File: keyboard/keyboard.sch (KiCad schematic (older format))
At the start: 356 parts, among them K1 KEYSW, K10 KEYSW, K100 KEYSW, K101 KEYSW, K102 KEYSW, K103 KEYSW, K104 KEYSW, K11 KEYSW, K12 KEYSW, K13 KEYSW, K14 KEYSW, K15 KEYSW, K16 KEYSW, K17 KEYSW, K18 KEYSW, K19 KEYSW, K2 KEYSW, K20 KEYSW, K21 KEYSW, K22 KEYSW, K23 KEYSW, K24 KEYSW, K25 KEYSW, K26 KEYSW, K27 KEYSW, K28 KEYSW, K29 KEYSW, K3 KEYSW, K30 KEYSW, K31 KEYSW, K32 KEYSW, K33 KEYSW, K34 KEYSW, K35 KEYSW, K36 KEYSW, K37 KEYSW, K38 KEYSW, K39 KEYSW, K4 KEYSW, K40 KEYSW, K41 KEYSW, K42 KEYSW, K43 KEYSW, K44 KEYSW, K45 KEYSW, K46 KEYSW, K47 KEYSW, K48 KEYSW, K49 KEYSW, K5 KEYSW, K50 KEYSW, K51 KEYSW, K52 KEYSW, K53 KEYSW, K54 KEYSW, K55 KEYSW, K56 KEYSW, K57 KEYSW, K58 KEYSW, K59 KEYSW, K6 KEYSW, K60 KEYSW, K61 KEYSW, K62 KEYSW, K63 KEYSW, K64 KEYSW, K65 KEYSW, K66 KEYSW, K67 KEYSW, K68 KEYSW, K69 KEYSW, K7 KEYSW, K70 KEYSW, K71 KEYSW, K72 KEYSW, K73 KEYSW, K74 KEYSW, K75 KEYSW, K76 KEYSW, K77 KEYSW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

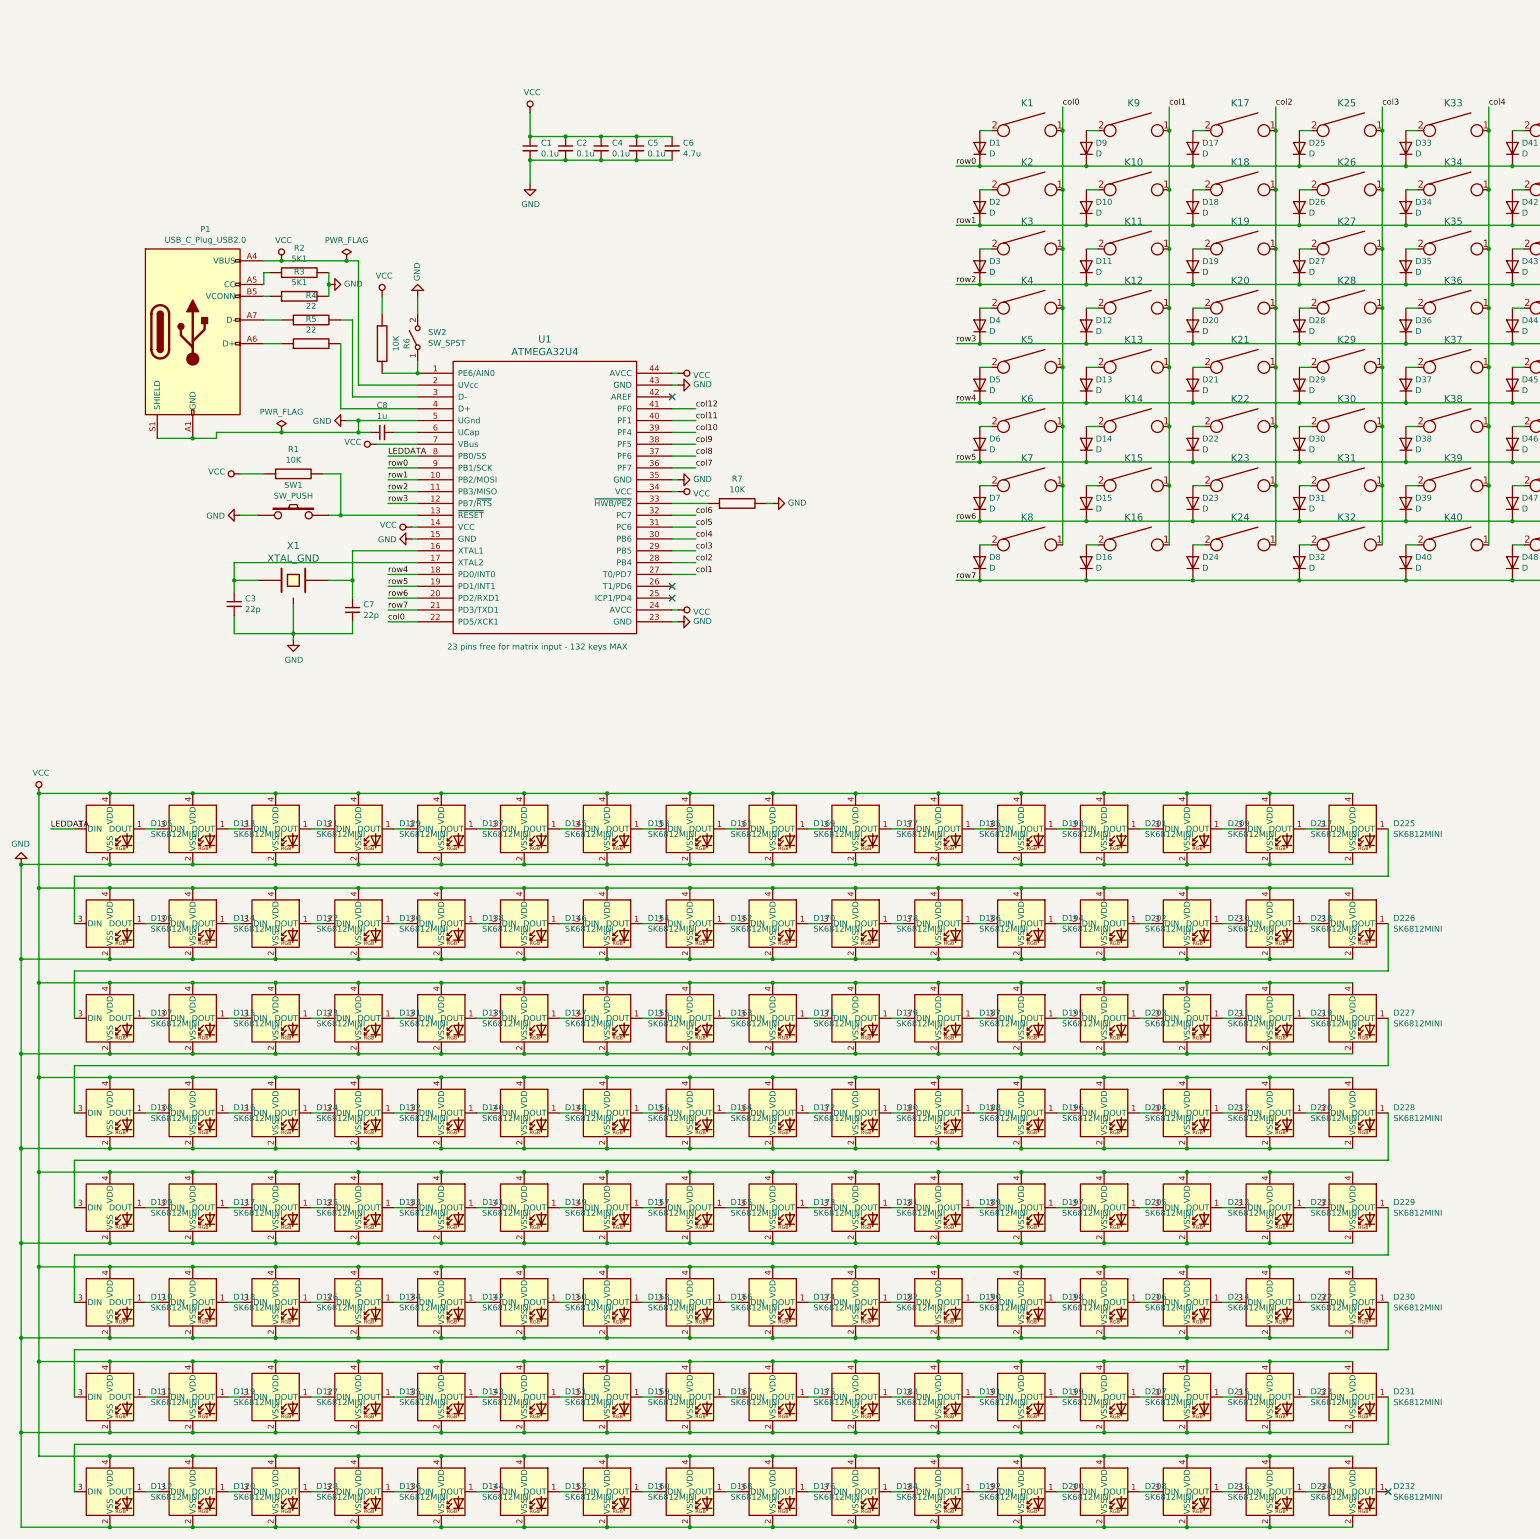
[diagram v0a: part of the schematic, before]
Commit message: add datasheets
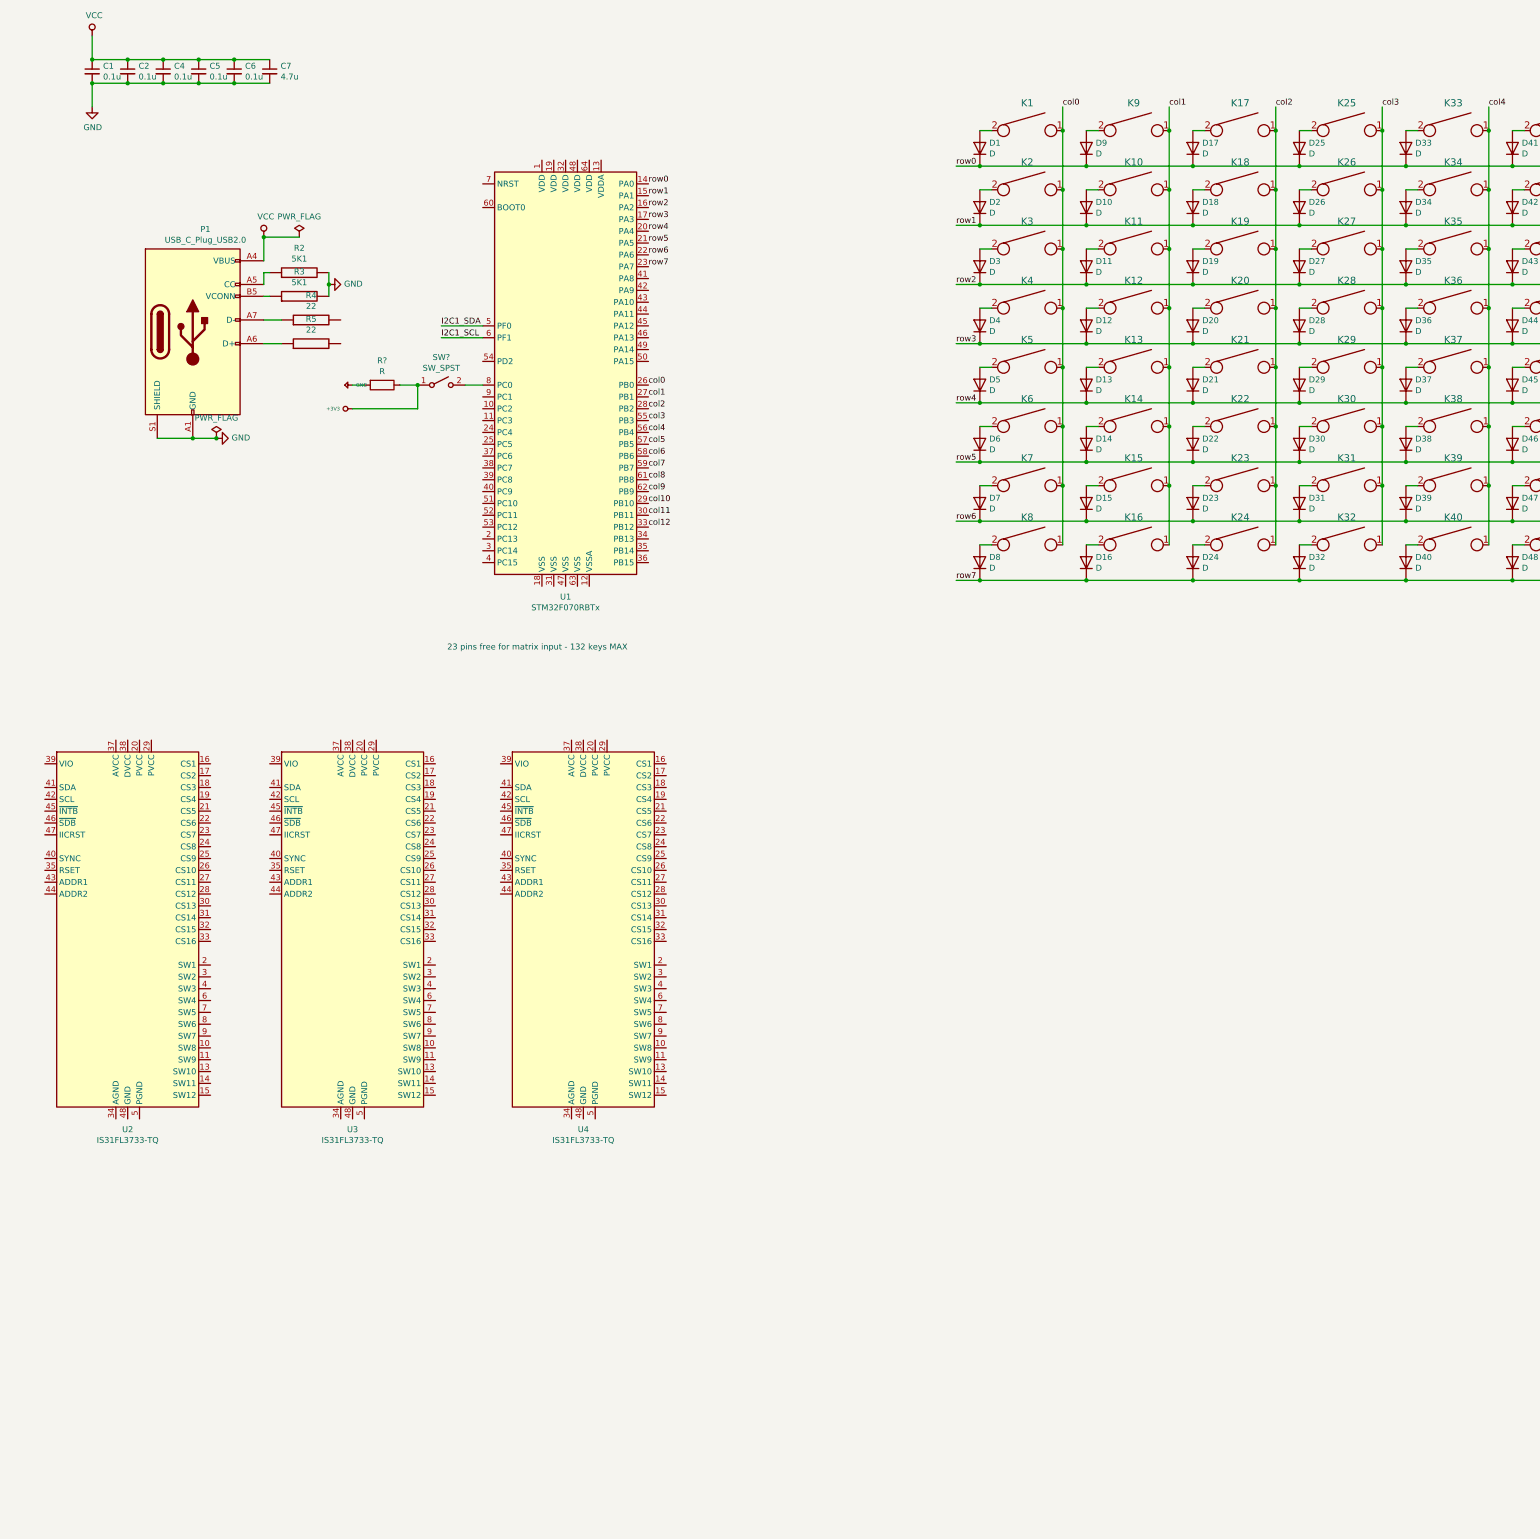
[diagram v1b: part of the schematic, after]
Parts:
- removed C3, C7: 22p, Capacitor_SMD:C_0805_2012Metric, symbol Device:C_Small
- removed C8: 1u, Capacitor_SMD:C_0805_2012Metric, symbol Device:C_Small
- removed D105, D106, D107, D108, D109, D110, D111, D112, D113, D114, D115, D116, D117, D118, D119, D120, D121, D122, D123, D124, D125, D126, D127, D128, D129, D130, D131, D132, D133, D134, D135, D136, D137, D138, D139, D140, D141, D142, D143, D144, D145, D146, D147, D148, D149, D150, D151, D152, D153, D154, D155, D156, D157, D158, D159, D160, D161, D162, D163, D164, D165, D166, D167, D168, D169, D170, D171, D172, D173, D174, D175, D176, D177, D178, D179, D180, D181, D182, D183, D184, D185, D186, D187, D188, D189, D190, D191, D192, D193, D194, D195, D196, D197, D198, D199, D200, D201, D202, D203, D204, D205, D206, D207, D208, D209, D210, D211, D212, D213, D214, D215, D216, D217, D218, D219, D220, D221, D222, D223, D224, D225, D226, D227, D228, D229, D230, D231, D232: SK6812MINI, LED_SMD:LED_SK6812MINI_PLCC4_3.5x3.5mm_P1.75mm, symbol LED:SK6812MINI
- removed R1, R6, R7: 10K, Resistor_SMD:R_0805_2012Metric, symbol keyboard:R
- removed SW1: SW_PUSH, Button_Switch_SMD:SW_SPST_TL3342, symbol keyboard:SW_PUSH
- removed SW2: SW_SPST, Button_Switch_THT:SW_Slide_1P2T_CK_OS102011MS2Q, symbol Switch:SW_SPST
- removed U1: ATMEGA32U4, Package_QFP:TQFP-44_10x10mm_P0.8mm, symbol keyboard:ATMEGA32U4
- removed X1: XTAL_GND, Crystal:Crystal_SMD_SeikoEpson_FA238-4Pin_3.2x2.5mm_HandSoldering, symbol keyboard:XTAL_GND
- added C6: 0.1u, symbol Device:C_Small
- added R?: R, symbol Device:R
- added SW?: SW_SPST, symbol Switch:SW_SPST
- added U1: STM32F070RBTx, Package_QFP:LQFP-64_10x10mm_P0.5mm, symbol MCU_ST_STM32F0:STM32F070RBTx
- added U2, U3, U4: IS31FL3733-TQ, Package_QFP:TQFP-48-1EP_7x7mm_P0.5mm_EP5x5mm, symbol Driver_LED:IS31FL3733-TQ
- renumbered C6 to C7
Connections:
- net GND: now also C6.2
- net VCC: now also C6.1
- net col0: now also U1.26 (PB0)
- net col1: now also U1.27 (PB1)
- net col10: now also U1.29 (PB10)
- net col11: now also U1.30 (PB11)
- net col12: now also U1.33 (PB12)
- net col2: now also U1.28 (PB2)
- net col3: now also U1.55 (PB3)
- net col4: now also U1.56 (PB4)
- net col5: now also U1.57 (PB5)
- net col6: now also U1.58 (PB6)
- net col7: now also U1.59 (PB7)
- net col8: now also U1.61 (PB8)
- net col9: now also U1.62 (PB9)
- net row0: now also U1.14 (PA0)
- net row1: now also U1.15 (PA1)
- net row2: now also U1.16 (PA2)
- net row3: now also U1.17 (PA3)
- net row4: now also U1.20 (PA4)
- net row5: now also U1.21 (PA5)
- net row6: now also U1.22 (PA6)
- net row7: now also U1.23 (PA7)
- new net: SW?.2 (B), U1.8 (PC0)
- new net: U2.12 (PGND), U2.5 (PGND)
- new net: U2.48 (GND), U2.49 (GND)
- new net: U3.12 (PGND), U3.5 (PGND)
- new net: U3.48 (GND), U3.49 (GND)
- new net: U4.12 (PGND), U4.5 (PGND)
- new net: U4.48 (GND), U4.49 (GND)
- new net +5V: R?.1, R?.2, SW?.1 (A)
- new net I2C1_SCL: U1.6 (PF1)
- new net I2C1_SDA: U1.5 (PF0)
- no-connect marks 4 -> 0
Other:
- moved on the sheet: C1, C2, C4, C5, C7
